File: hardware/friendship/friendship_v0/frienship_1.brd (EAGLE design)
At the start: 100 x 80 mm, 25 parts, among them T1 BCX70SMD, T2 BCX70SMD, T3 BCX70SMD, T4 BCX70SMD

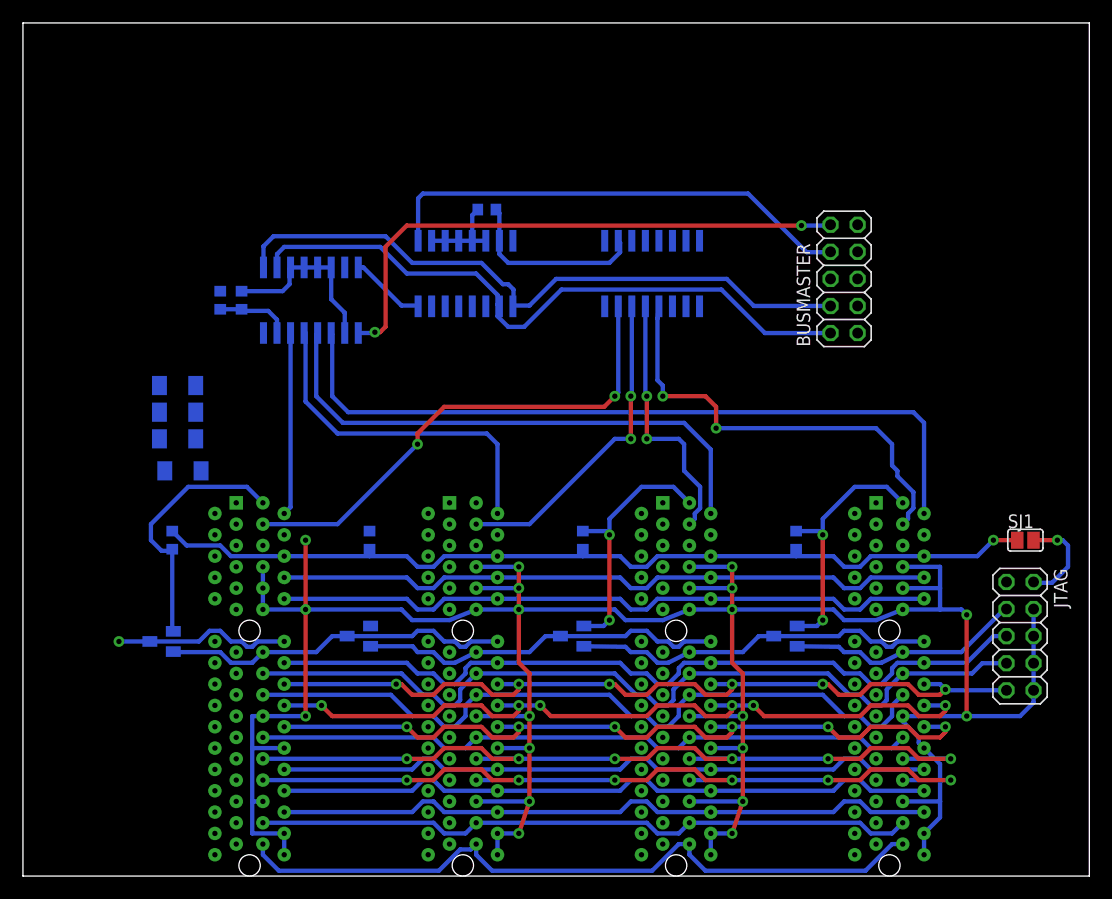
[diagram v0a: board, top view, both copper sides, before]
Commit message: moar awesome
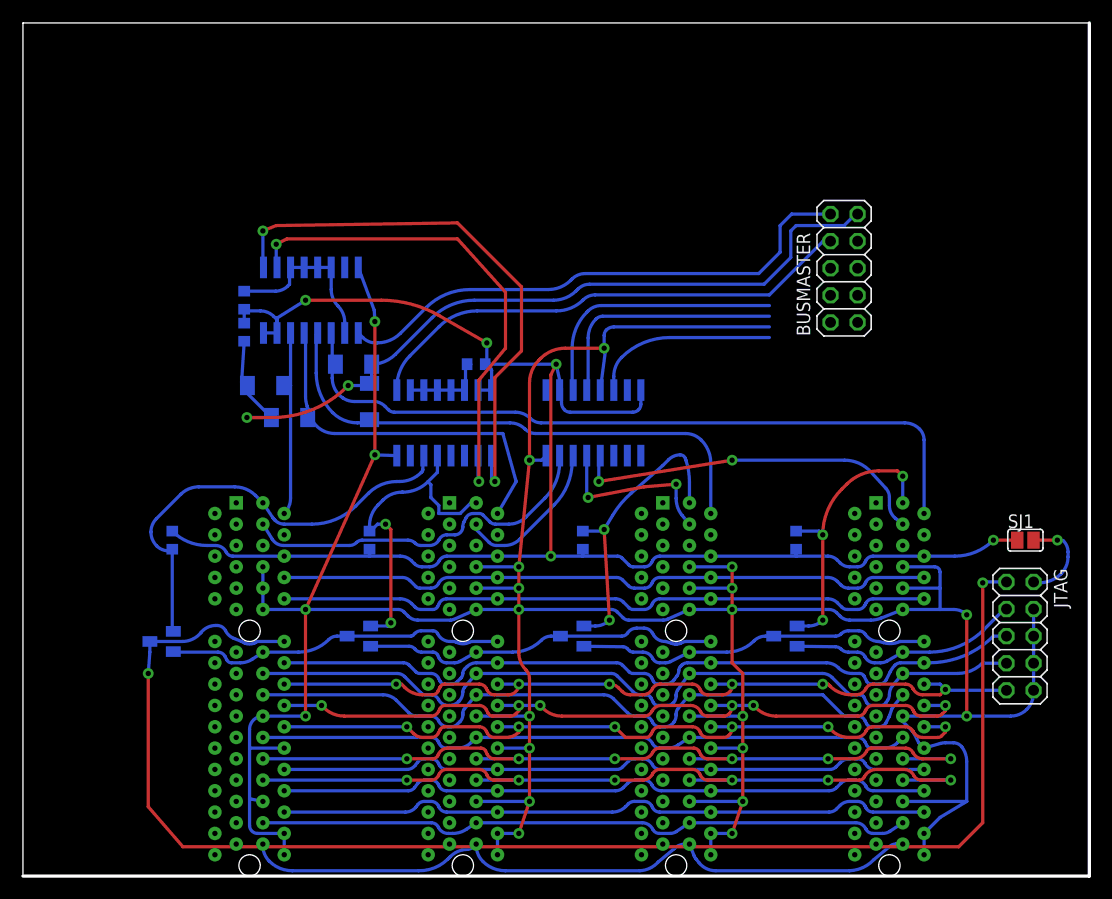
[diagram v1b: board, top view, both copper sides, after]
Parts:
- moved D1 18.9 mm to (31.0, 48.0), turned to 180 degrees
- moved D4 18.3 mm to (32.5, 44.5), turned to 90 degrees
- moved INTACK_LATCH 15.0 mm to (53.5, 42.5)
- moved R12 14.5 mm to (42.5, 48.0)
- moved PRSNT_LATCH 14.1 mm to (39.5, 42.5)
- moved D2 10.5 mm to (25.0, 43.0)
- moved D3 8.25 mm to (22.8, 46.0)
- moved R5 3.75 mm to (20.8, 51.0), turned to 90 degrees
- moved BUSMASTER 1.00 mm to (77.0, 57.0)
- moved R7 0.25 mm to (20.8, 54.0)
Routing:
- net TDI: track 16.7 -> 134.6 mm, vias 1 -> 2
- net N$11: track 0.00 -> 76.9 mm, vias 0 -> 2
- net GND: track 282.4 -> 359.1 mm, vias 19 -> 22
- net 3V3: track 109.8 -> 158.6 mm, vias 1 -> 5
- net PRSNT1: track 0.00 -> 31.2 mm, vias 0 -> 2
- net N$4: track 0.00 -> 24.9 mm
- net N$9: track 0.00 -> 23.2 mm
- net PRSNT0: track 24.3 -> 42.3 mm
- net N$1: track 0.00 -> 17.4 mm
- net /CS1: track 30.3 -> 15.0 mm, vias 2 -> 0
- net SHIFT: track 61.0 -> 47.2 mm, vias 0 -> 2
- net /CS0: track 47.1 -> 34.4 mm, vias 2 -> 0
- net N$3: track 61.4 -> 52.1 mm, vias 0 -> 2
- net /CS2: track 24.7 -> 16.4 mm
- net /CS3: track 41.9 -> 34.4 mm
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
